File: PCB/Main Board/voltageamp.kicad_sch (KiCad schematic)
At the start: 47 parts, among them U901 OPA2197xD, U902 INA828D, U903 DG201, U904 DG201, U905 OPA2197xD

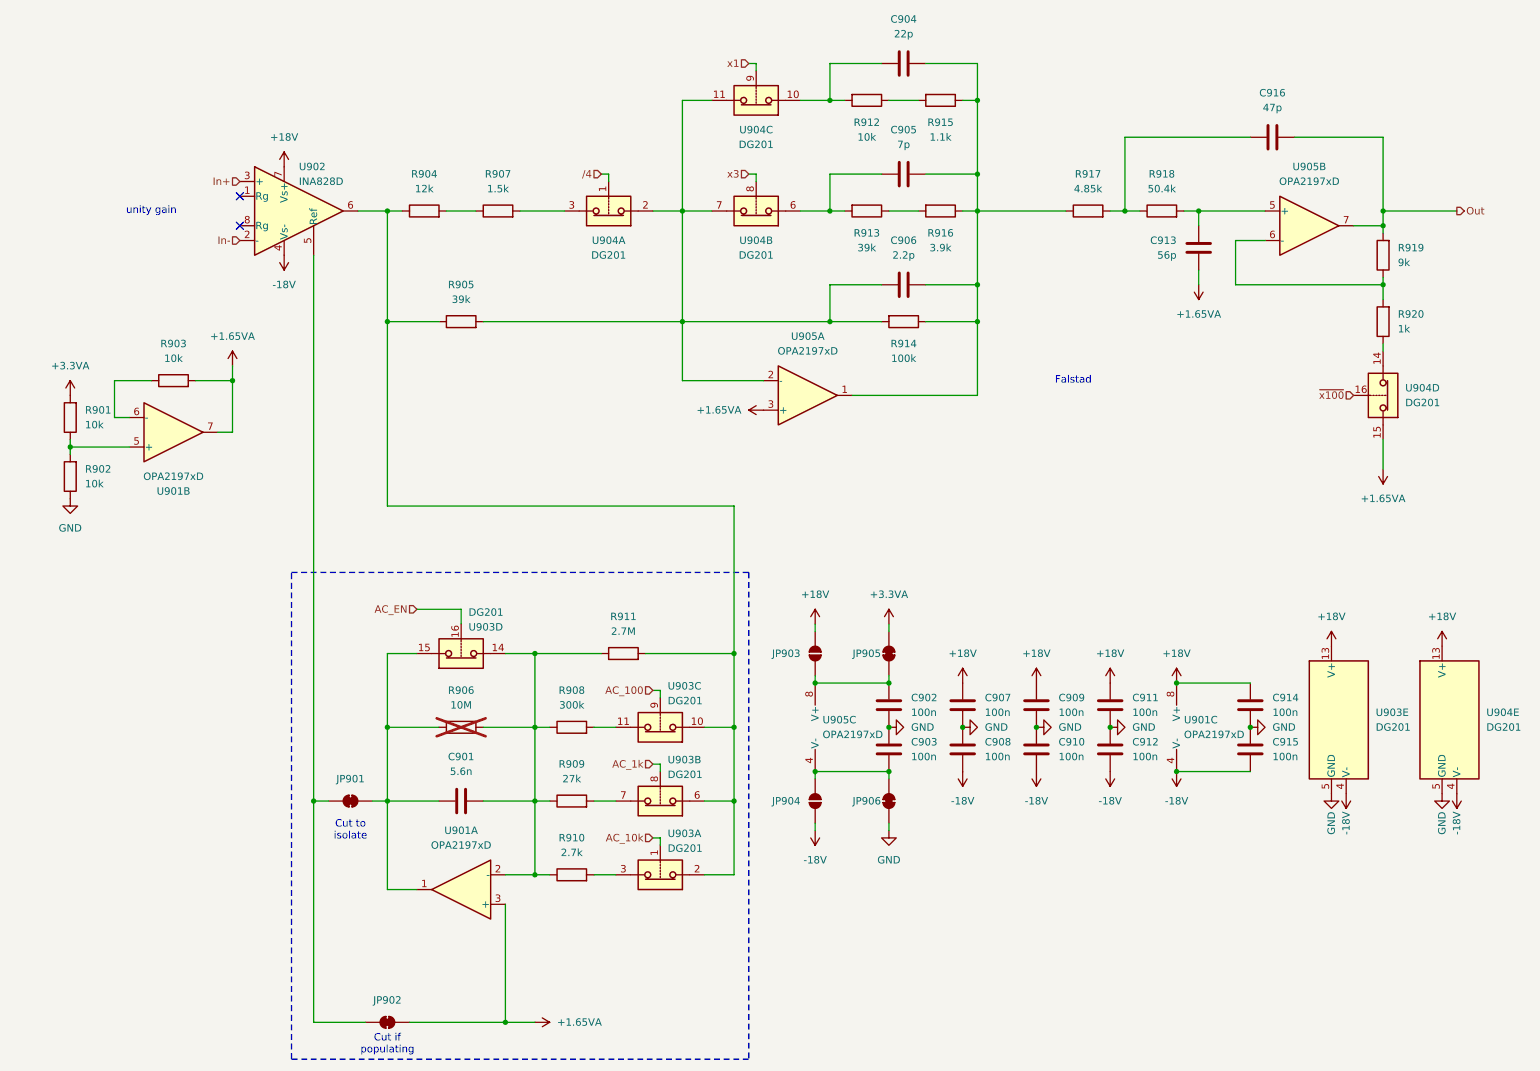
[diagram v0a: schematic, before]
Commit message: Layout progress
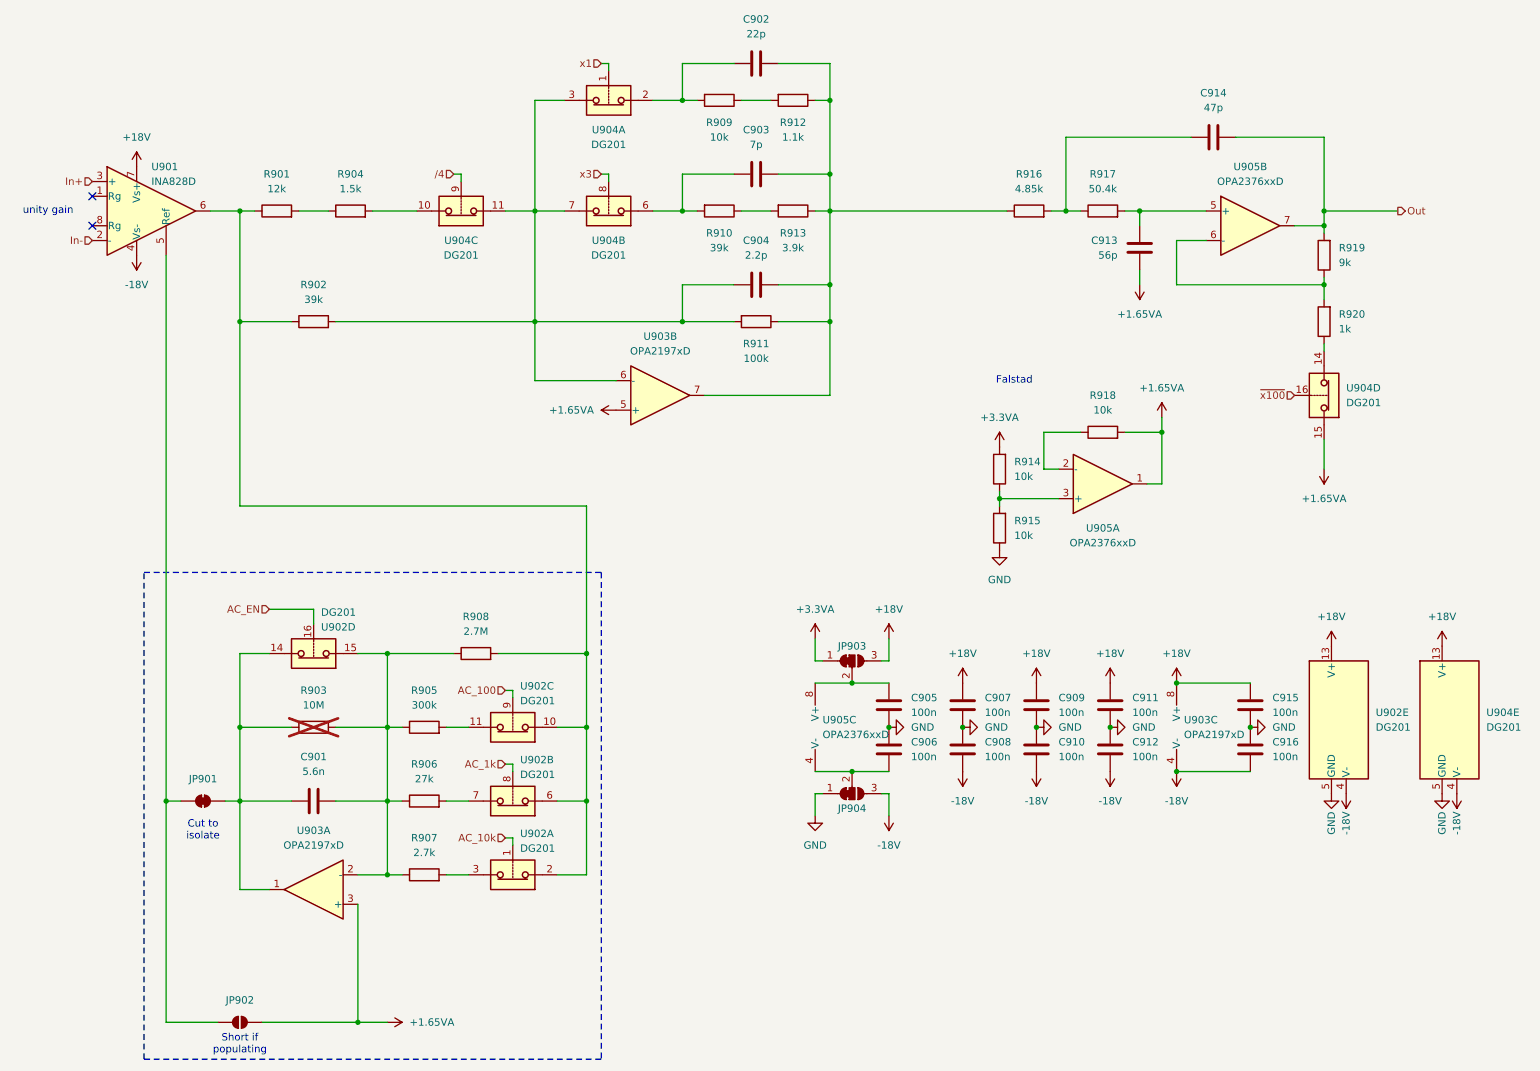
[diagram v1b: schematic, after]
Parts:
- removed JP902, JP905, JP906: SolderJumper_2_Bridged, Jumper:SolderJumper-2_P1.3mm_Bridged_RoundedPad1.0x1.5mm, symbol Jumper:SolderJumper_2_Bridged
- removed JP903, JP904: SolderJumper_2_Open, Jumper:SolderJumper-2_P1.3mm_Open_RoundedPad1.0x1.5mm, symbol Jumper:SolderJumper_2_Open
- removed unit 2 of U901
- removed unit 2 of U905
- removed unit 3 of U905
- added JP902: SolderJumper_2_Open, Jumper:SolderJumper-2_P1.3mm_Open_RoundedPad1.0x1.5mm, symbol Jumper:SolderJumper_2_Open
- added JP903, JP904: SolderJumper_3_Bridged12, Jumper:SolderJumper-3_P1.3mm_Bridged123_RoundedPad1.0x1.5mm, symbol Jumper:SolderJumper_3_Bridged12
- added U905: OPA2376xxD, Package_SO:SOIC-8_3.9x4.9mm_P1.27mm, symbol Amplifier_Operational:OPA2376xxD
- renumbered C904 to C902, C905 to C903, C906 to C904, C902 to C905, C903 to C906, C916 to C914, C914 to C915, C915 to C916, R904 to R901, R905 to R902, R906 to R903, R907 to R904, R908 to R905, R909 to R906, R910 to R907, R911 to R908, R912 to R909, R913 to R910, R914 to R911, R915 to R912, R916 to R913, R901 to R914, R902 to R915, R917 to R916, R918 to R917, R903 to R918, U902 to U901, U903 to U902, U901 to U903, U905 to U903
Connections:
- net +1.65VA: now also U903.5 (+), JP902.2 (B), U905.1; no longer U903.3 (+)
- net +18V: now also JP903.3 (B)
- net +3.3VA: now also JP903.1 (A)
- net -18V: now also JP904.3 (B)
- net GND: now also JP904.1 (A)
- net Out: now also U905.7
- net x1: now also U904.1; no longer U904.9
- net /4: now also U904.9; no longer U904.1
- net at C901.2, R903.2, R905.1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: now also U902.15; no longer U902.14
- net at C901.1, JP901.2 (B), R903.1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: now also U902.14; no longer U902.15
- net at C904.1, R902.2, R911.2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: now also U903.6 (-), U904.3; no longer U903.2 (-), U904.2
- net at C902.2, C903.2, C904.2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: now also U903.7; no longer U903.1
- net at R904.2: now also U904.10; no longer U904.3
- net at C906.2: now also JP904.2 (C), U905.4 (V-)
- net at C902.1, R909.2: now also U904.2; no longer U904.10
- net at R919.1, R920.2: now also U905.6 (-)
- net at R914.1, R915.2: now also U905.3 (+)
- net at R918.1: now also U905.2 (-)
- net at C913.1, R917.2: now also U905.5 (+)
- net at JP901.1 (A), U901.5 (Ref): now also JP902.1 (A)
- net at C905.1: now also JP903.2 (C), U905.8 (V+)
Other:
- note added: "Short if populating"
- note removed: "Cut if populating"
- moved on the sheet: C901, C902, C903, C904, C913, C914, JP901, R901, R902, R903, R904, R905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
